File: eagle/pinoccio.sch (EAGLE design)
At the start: 51 parts, among them Q1 16MHz, Q2 32.768k, Q4 MOSFET-PCHANNEL, Q5 TRANSISTOR-NPN-DUAL, U1 MCP73831, U2 3.3V, U4 ATMEGA128RFA1, X1 USB-MICROB, Y2 ANTENNA2SMD5

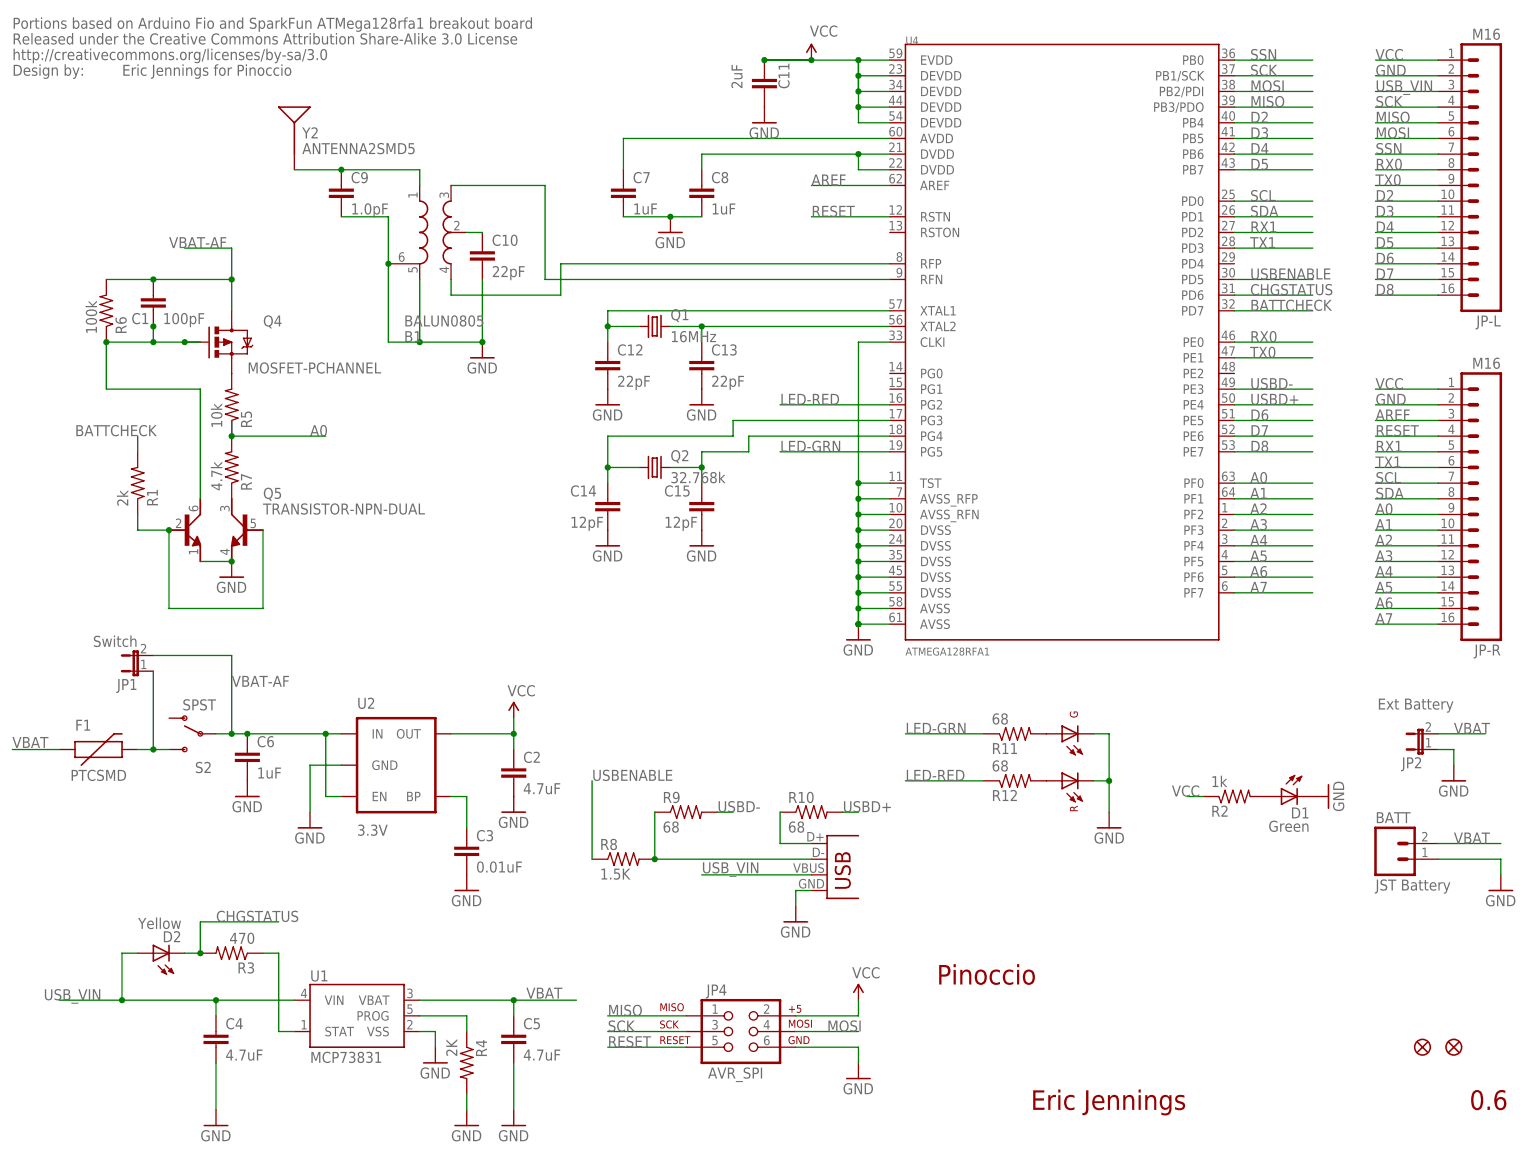
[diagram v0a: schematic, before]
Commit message: Update licensing on eagle files
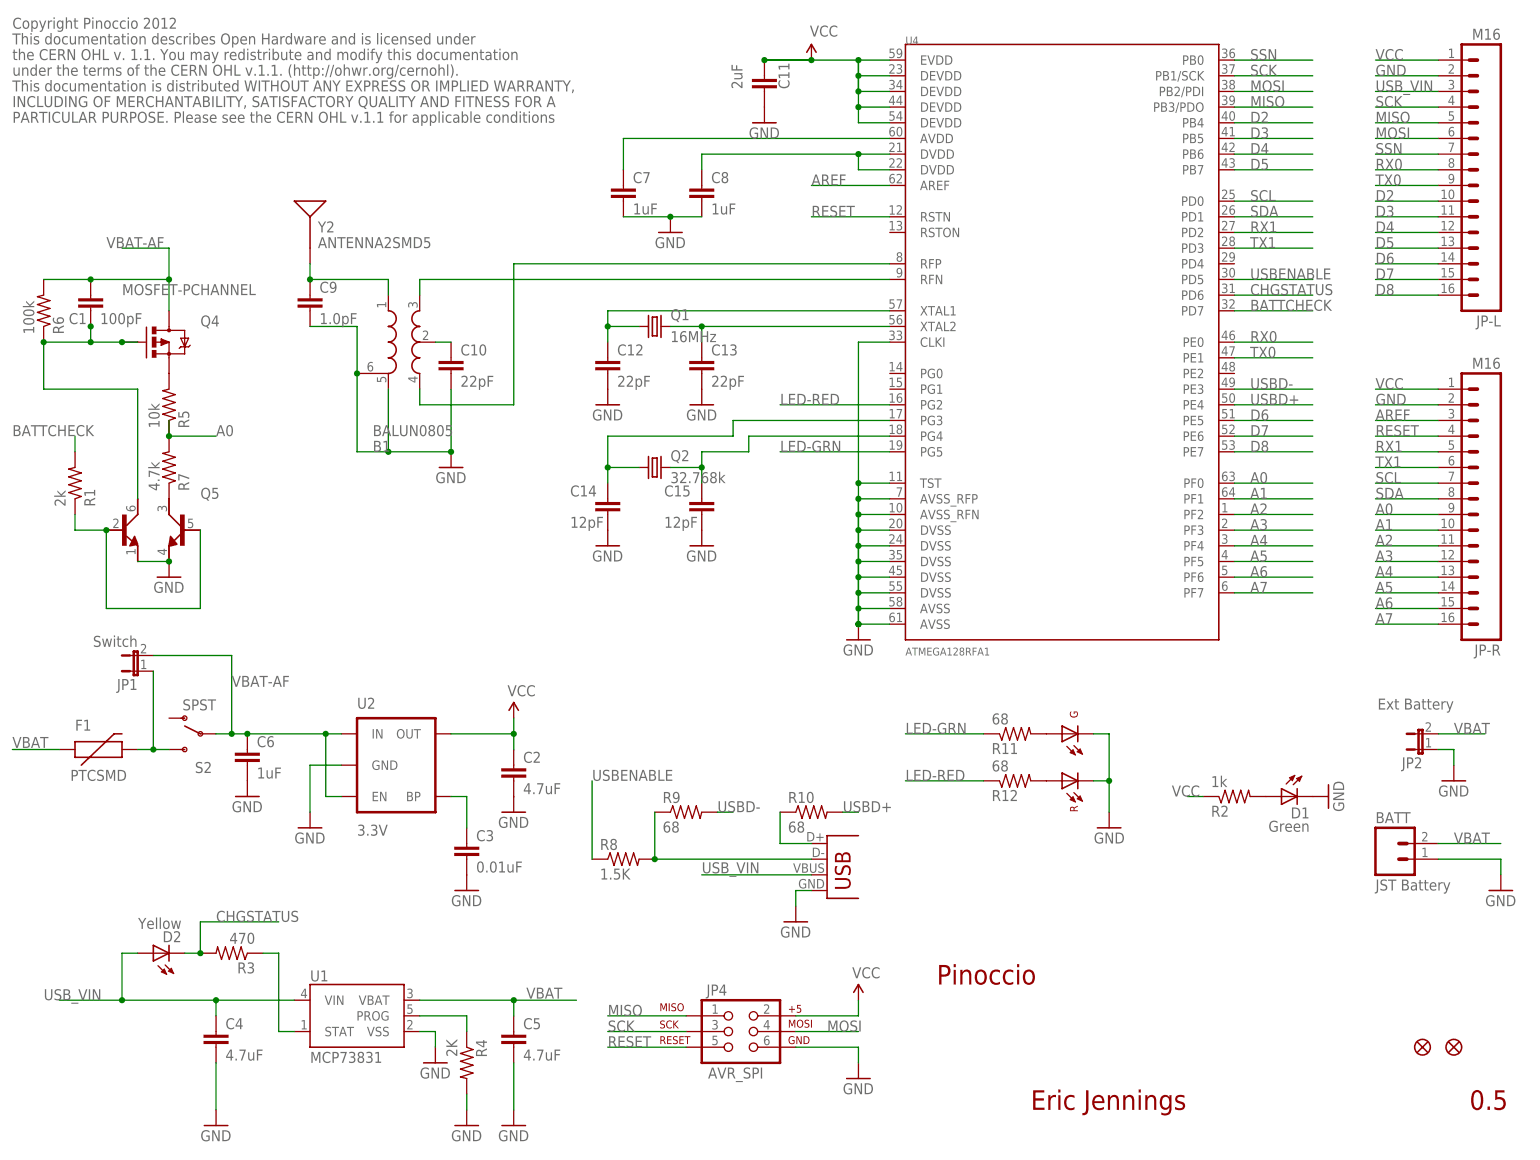
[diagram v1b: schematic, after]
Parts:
- removed U$3: CREATIVE_COMMONS, SparkFun:CREATIVE_COMMONS
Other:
- note added: "0.5"
- note added: "Copyright Pinoccio 2012"
- note added: "INCLUDING OF MERCHANTABILITY, SATISFACTORY QUALITY AND FITNESS FOR A"
- note added: "PARTICULAR PURPOSE. Please see the CERN OHL v.1.1 for applicable conditions"
- note added: "This documentation describes Open Hardware and is licensed under"
- note added: "This documentation is distributed WITHOUT ANY EXPRESS OR IMPLIED WARRANTY,"
- note added: "the CERN OHL v. 1.1. You may redistribute and modify this documentation"
- note added: "under the terms of the CERN OHL v.1.1. (http://ohwr.org/cernohl)."
- note removed: "0.6"
- note removed: "Eric Jennings for Pinoccio"
- note removed: "Portions based on Arduino Fio and SparkFun ATMega128rfa1 breakout board"
- moved on the sheet: B1, C1, C10, C9, Q4, Q5, R1, R5, R6, R7, Y2
